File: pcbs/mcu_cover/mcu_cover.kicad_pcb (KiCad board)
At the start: 2 copper layers, 19.4 x 56.7 mm, 2 parts

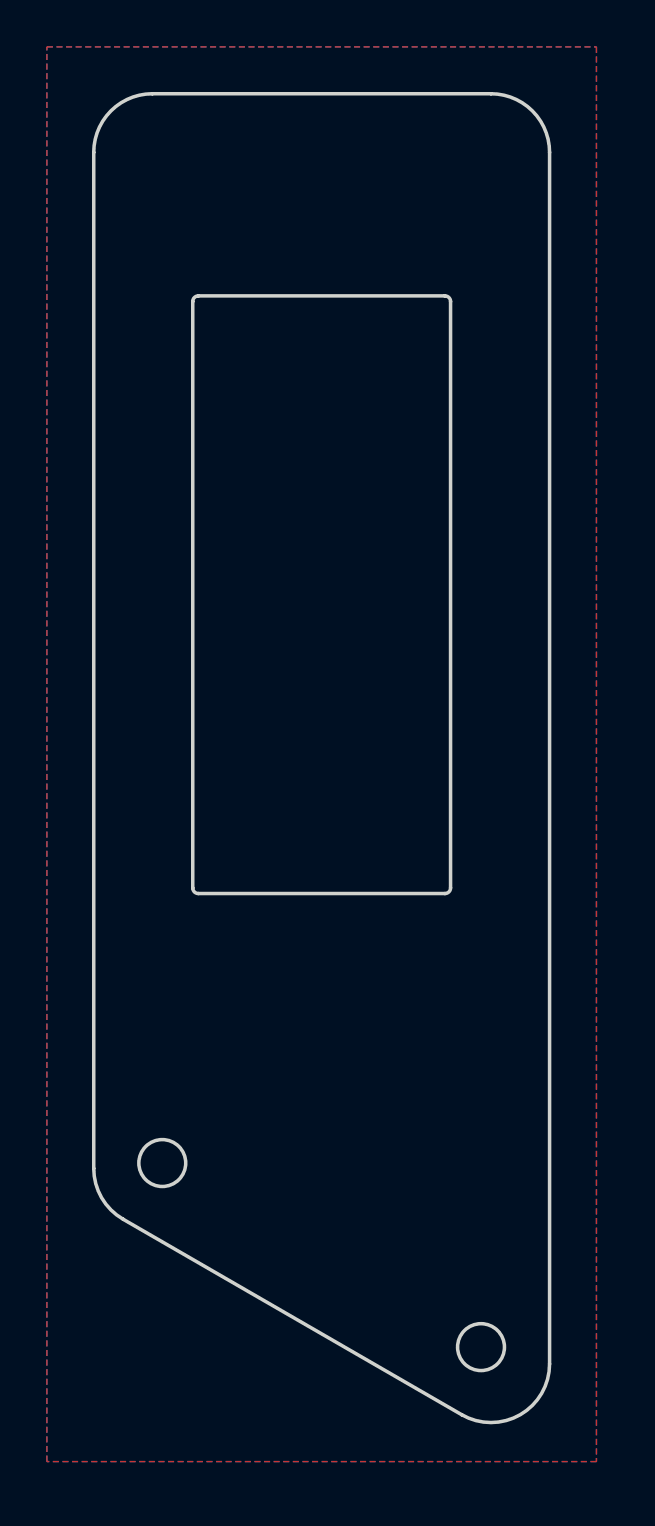
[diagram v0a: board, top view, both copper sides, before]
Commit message: update naming and gen files
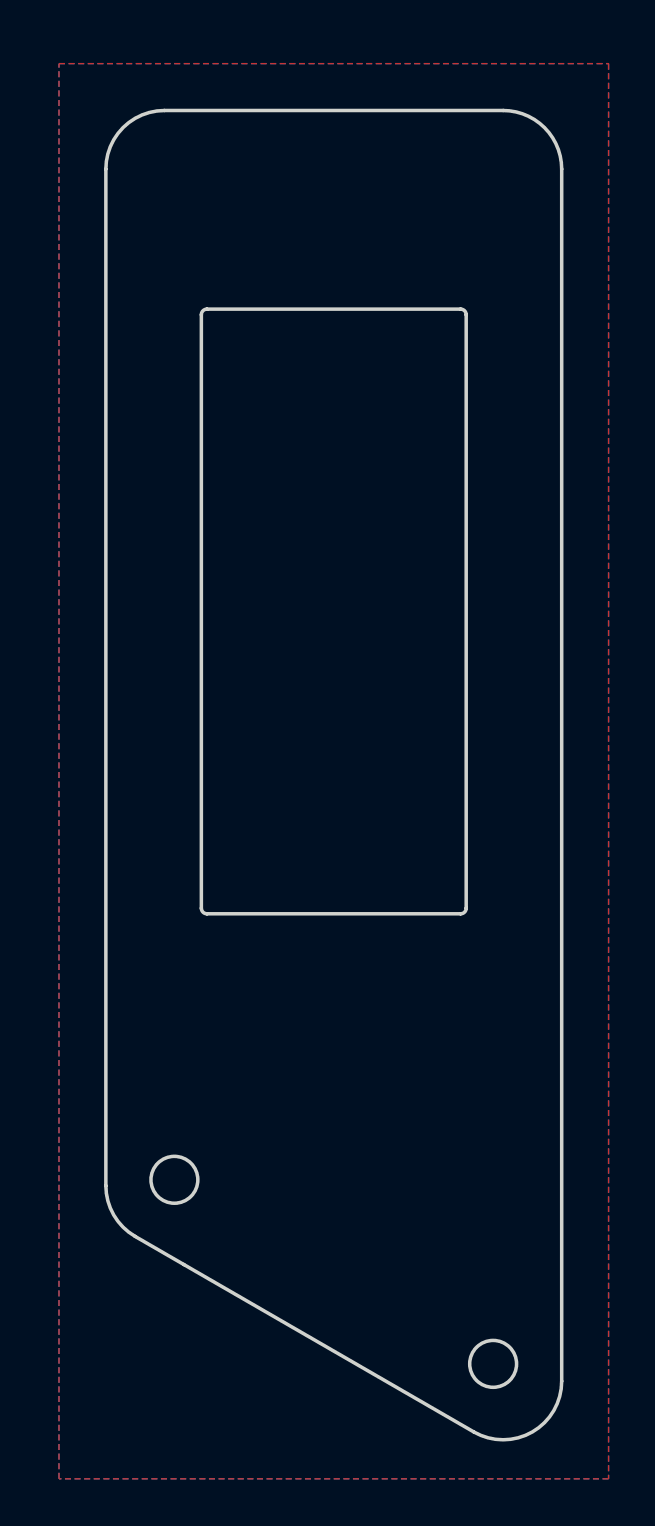
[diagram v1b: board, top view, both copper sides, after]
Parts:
- moved MH2 0.88 mm to (163.5, 95.3)
- moved MH1 0.88 mm to (149.9, 87.4)
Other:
- outline, holes or cut-outs redrawn
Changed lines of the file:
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@@
 	(title_block
 		(title "mcu_cover")
-		(date "2025-11-30")
+		(date "2025-12-13")
 		(rev "1")
 		(company "Curtis Bollinger")
@@
 	(footprint "ceoloide:mounting_hole_npth"
 		(layer "F.Cu")
-		(at 149.422875 86.721437)
-		(property "Reference" "MH1"
+		(at 163.539872 95.289966)
+		(property "Reference" "MH2"
 			(at 0 2.55 0)
 			(layer "F.SilkS")
@@
 	(footprint "ceoloide:mounting_hole_npth"
 		(layer "F.Cu")
-		(at 163.022875 94.575437)
-		(property "Reference" "MH2"
+		(at 149.939872 87.435966)
+		(property "Reference" "MH1"
 			(at 0 2.55 0)
 			(layer "F.SilkS")
@@
 		(embedded_fonts no)
 	)
-	(gr_arc
-		(start 150.962875 75.221437)
-		(mid 150.793172 75.151136)
-		(end 150.722875 74.981437)
-		(stroke
-			(width 0.15)
-			(type default)
-		)
-		(layer "Edge.Cuts")
-	)
-	(gr_arc
-		(start 161.482875 49.721437)
-		(mid 161.652584 49.791725)
-		(end 161.722875 49.961437)
-		(stroke
-			(width 0.15)
-			(type default)
-		)
-		(layer "Edge.Cuts")
-	)
-	(gr_line
-		(start 150.962875 75.221437)
-		(end 161.482875 75.221437)
-		(stroke
-			(width 0.15)
-			(type default)
-		)
-		(layer "Edge.Cuts")
-	)
-	(gr_line
-		(start 161.482875 49.721437)
-		(end 150.962875 49.721437)
+	(gr_line
+		(start 163.964872 41.810966)
+		(end 149.515372 41.810966)
 		(stroke
 			(width 0.15)
@@
 	)
 	(gr_circle
-		(center 149.422875 86.721437)
-		(end 150.422875 86.721437)
+		(center 149.939872 87.435966)
+		(end 150.939872 87.435966)
 		(stroke
 			(width 0.15)
@@
 		(layer "Edge.Cuts")
 	)
-	(gr_line
-		(start 165.947875 95.293974)
-		(end 165.947875 43.596437)
-		(stroke
-			(width 0.15)
-			(type default)
-		)
-		(layer "Edge.Cuts")
-	)
-	(gr_line
-		(start 150.722875 49.961437)
-		(end 150.722875 74.981437)
-		(stroke
-			(width 0.15)
-			(type default)
-		)
-		(layer "Edge.Cuts")
-	)
-	(gr_line
-		(start 163.447875 41.096437)
-		(end 148.998375 41.096437)
-		(stroke
-			(width 0.15)
-			(type default)
-		)
-		(layer "Edge.Cuts")
-	)
-	(gr_arc
-		(start 163.447875 41.096437)
-		(mid 165.215645 41.828663)
-		(end 165.947875 43.596437)
-		(stroke
-			(width 0.15)
-			(type default)
-		)
-		(layer "Edge.Cuts")
-	)
-	(gr_line
-		(start 146.498375 86.951552)
-		(end 146.498375 43.596437)
-		(stroke
-			(width 0.15)
-			(type default)
-		)
-		(layer "Edge.Cuts")
-	)
-	(gr_line
-		(start 147.748375 89.116615)
-		(end 162.197875 97.459038)
-		(stroke
-			(width 0.15)
-			(type default)
-		)
-		(layer "Edge.Cuts")
-	)
-	(gr_arc
-		(start 165.947875 95.293974)
-		(mid 164.697859 97.458972)
-		(end 162.197875 97.459038)
-		(stroke
-			(width 0.15)
-			(type default)
-		)
-		(layer "Edge.Cuts")
-	)
-	(gr_arc
-		(start 150.722875 49.961437)
-		(mid 150.793155 49.791699)
-		(end 150.962875 49.721437)
-		(stroke
-			(width 0.15)
-			(type default)
-		)
-		(layer "Edge.Cuts")
-	)
-	(gr_arc
-		(start 147.748375 89.116615)
-		(mid 146.833339 88.201545)
-		(end 146.498375 86.951552)
-		(stroke
-			(width 0.15)
-			(type default)
-		)
-		(layer "Edge.Cuts")
-	)
-	(gr_line
-		(start 161.722875 74.981437)
-		(end 161.722875 49.961437)
-		(stroke
-			(width 0.15)
-			(type default)
-		)
-		(layer "Edge.Cuts")
-	)
-	(gr_arc
-		(start 161.722875 74.981437)
-		(mid 161.652566 75.15111)
-		(end 161.482875 75.221437)
+	(gr_arc
+		(start 151.329872 76.085966)
+		(mid 151.160196 76.01566)
+		(end 151.089872 75.845966)
+		(stroke
+			(width 0.15)
+			(type default)
+		)
+		(layer "Edge.Cuts")
+	)
+	(gr_arc
+		(start 147.015372 44.310966)
+		(mid 147.747615 42.543211)
+		(end 149.515372 41.810966)
+		(stroke
+			(width 0.15)
+			(type default)
+		)
+		(layer "Edge.Cuts")
+	)
+	(gr_arc
+		(start 166.464872 96.029406)
+		(mid 165.214856 98.194404)
+		(end 162.714872 98.19447)
+		(stroke
+			(width 0.15)
+			(type default)
+		)
+		(layer "Edge.Cuts")
+	)
+	(gr_arc
+		(start 151.089872 50.525966)
+		(mid 151.160177 50.356272)
+		(end 151.329872 50.285966)
+		(stroke
+			(width 0.15)
+			(type default)
+		)
+		(layer "Edge.Cuts")
+	)
+	(gr_arc
+		(start 162.389872 75.845966)
+		(mid 162.319588 76.015684)
+		(end 162.149872 76.085966)
+		(stroke
+			(width 0.15)
+			(type default)
+		)
+		(layer "Edge.Cuts")
+	)
+	(gr_line
+		(start 162.714872 98.19447)
+		(end 150.343677 91.051957)
+		(stroke
+			(width 0.15)
+			(type default)
+		)
+		(layer "Edge.Cuts")
+	)
+	(gr_line
+		(start 147.015372 87.687099)
+		(end 147.015372 44.310966)
+		(stroke
+			(width 0.15)
+			(type default)
+		)
+		(layer "Edge.Cuts")
+	)
+	(gr_arc
+		(start 148.265372 89.852163)
+		(mid 147.350318 88.937096)
+		(end 147.015372 87.687099)
+		(stroke
+			(width 0.15)
+			(type default)
+		)
+		(layer "Edge.Cuts")
+	)
+	(gr_arc
+		(start 163.964872 41.810966)
+		(mid 165.732669 42.543187)
+		(end 166.464872 44.310966)
+		(stroke
+			(width 0.15)
+			(type default)
+		)
+		(layer "Edge.Cuts")
+	)
+	(gr_line
+		(start 148.265372 89.852163)
+		(end 150.343627 91.052044)
+		(stroke
+			(width 0.15)
+			(type default)
+		)
+		(layer "Edge.Cuts")
+	)
+	(gr_arc
+		(start 162.149872 50.285966)
+		(mid 162.319608 50.356248)
+		(end 162.389872 50.525966)
 		(stroke
 			(width 0.15)
@@
 	)
 	(gr_circle
-		(center 163.022875 94.575437)
-		(end 164.022875 94.575437)
+		(center 163.539872 95.289966)
+		(end 164.539872 95.289966)
 		(stroke
 			(width 0.15)
@@
 		(layer "Edge.Cuts")
 	)
-	(gr_arc
-		(start 146.498375 43.596437)
-		(mid 147.230593 41.828637)
-		(end 148.998375 41.096437)
+	(gr_line
+		(start 162.389872 75.845966)
+		(end 162.389872 50.525966)
+		(stroke
+			(width 0.15)
+			(type default)
+		)
+		(layer "Edge.Cuts")
+	)
+	(gr_line
+		(start 166.464872 96.029406)
+		(end 166.464872 44.310966)
+		(stroke
+			(width 0.15)
+			(type default)
+		)
+		(layer "Edge.Cuts")
+	)
+	(gr_line
+		(start 151.089872 50.525966)
+		(end 151.089872 75.845966)
+		(stroke
+			(width 0.15)
+			(type default)
+		)
+		(layer "Edge.Cuts")
+	)
+	(gr_line
+		(start 162.149872 50.285966)
+		(end 151.329872 50.285966)
+		(stroke
+			(width 0.15)
+			(type default)
+		)
+		(layer "Edge.Cuts")
+	)
+	(gr_line
+		(start 151.329872 76.085966)
+		(end 162.149872 76.085966)
 		(stroke
 			(width 0.15)
@@
 		(polygon
 			(pts
-				(xy 144.498375 39.096437) (xy 167.947875 39.096437) (xy 167.947875 99.459038) (xy 144.498375 99.459038)
+				(xy 145.015372 39.810966) (xy 168.464872 39.810966) (xy 168.464872 100.19447) (xy 145.015372 100.19447)
 			)
 		)
@@
 		(polygon
 			(pts
-				(xy 144.498375 39.096437) (xy 167.947875 39.096437) (xy 167.947875 99.459038) (xy 144.498375 99.459038)
-			)
-		)
+				(xy 145.015372 39.810966) (xy 168.464872 39.810966) (xy 168.464872 100.19447) (xy 145.015372 100.19447)
+			)
+		)
